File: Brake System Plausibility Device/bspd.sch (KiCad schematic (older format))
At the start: 22 parts, among them P1 Power_Entry, P2 5KW signal, P3 \"Hard_Braking\", P4 Q_AND_Q-NOT, SW1 RESET, U1 LM1117-5.0, U2 LM2903, U3 74LVC2G74

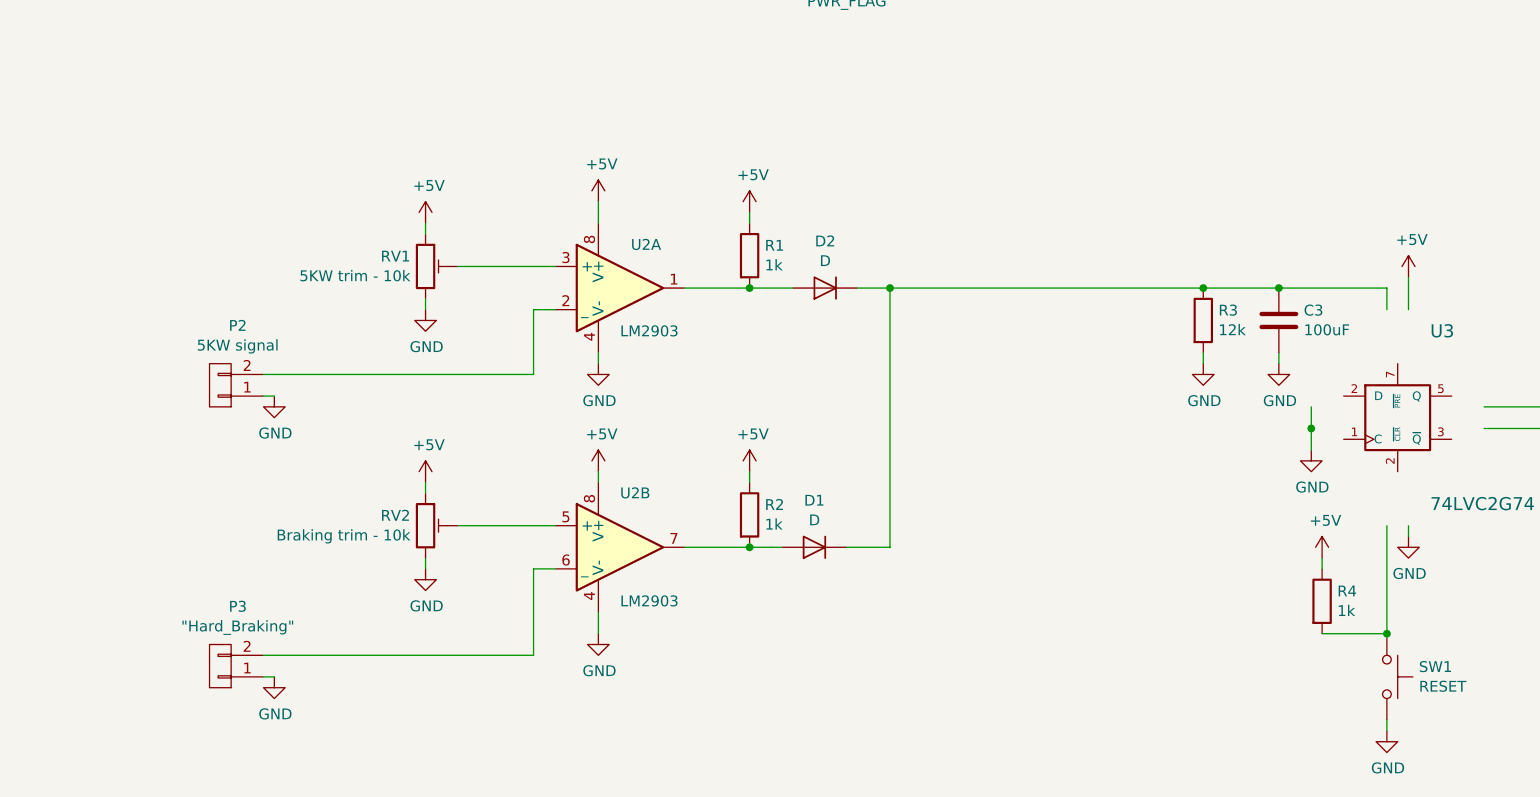
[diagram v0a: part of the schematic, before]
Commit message: Fix
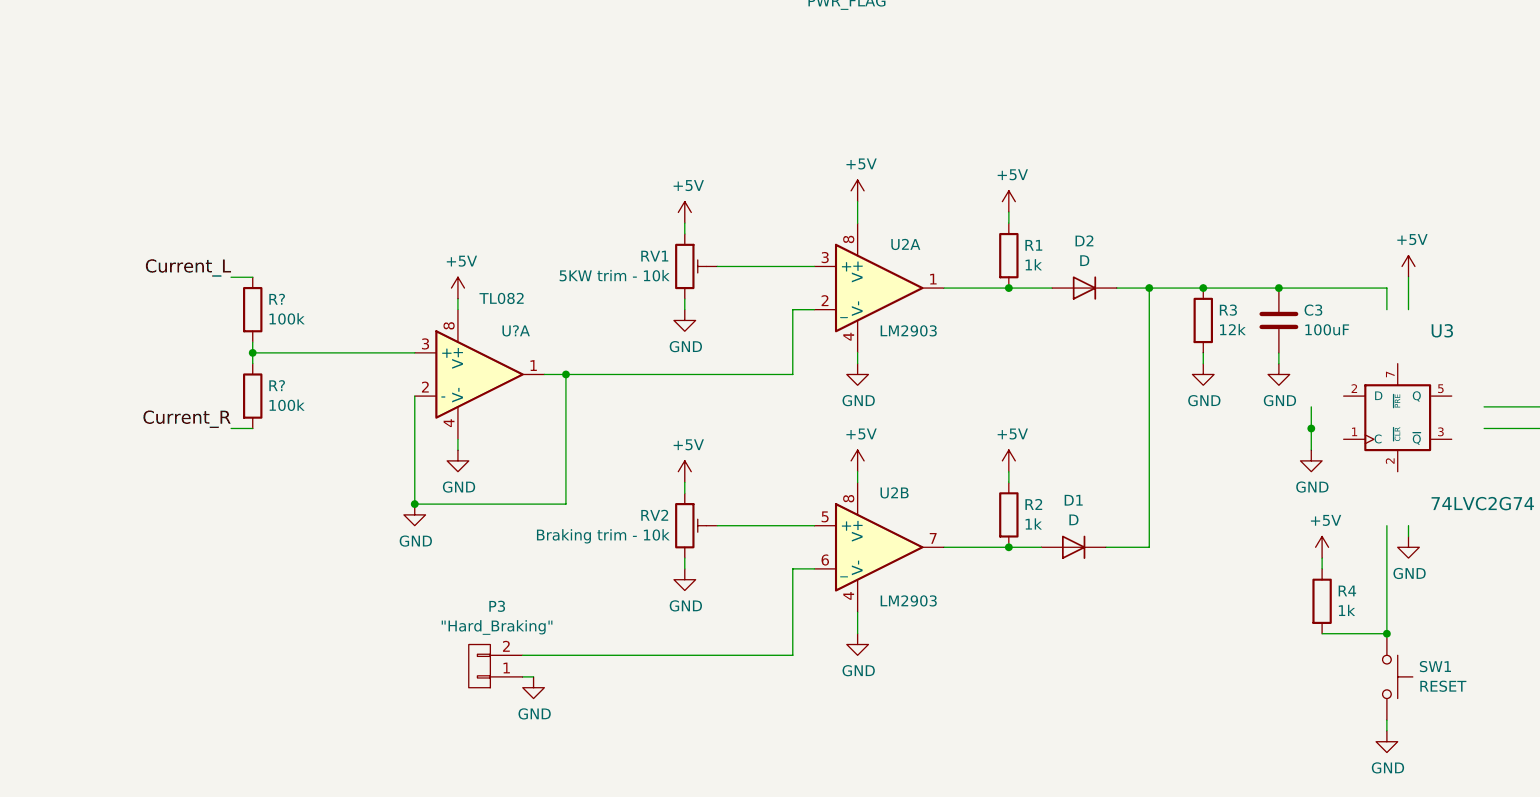
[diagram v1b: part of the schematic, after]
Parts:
- removed P2: 5KW signal, Pin_Headers:Pin_Header_Straight_1x02_Pitch2.54mm, symbol CONN_01X02
- added R? (x2): 100k, symbol R
- added U?: TL082, symbol TL082
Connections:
- net labels added: Current_L, Current_R
- wire segments 53 -> 61
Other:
- moved on the sheet: D1, D2, P3, R1, R2, RV1, RV2, U2A, U2B
